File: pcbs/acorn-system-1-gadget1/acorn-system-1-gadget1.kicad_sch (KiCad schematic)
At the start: 13 parts, among them J2 DIN41612_02x32_AB_acorn-syste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

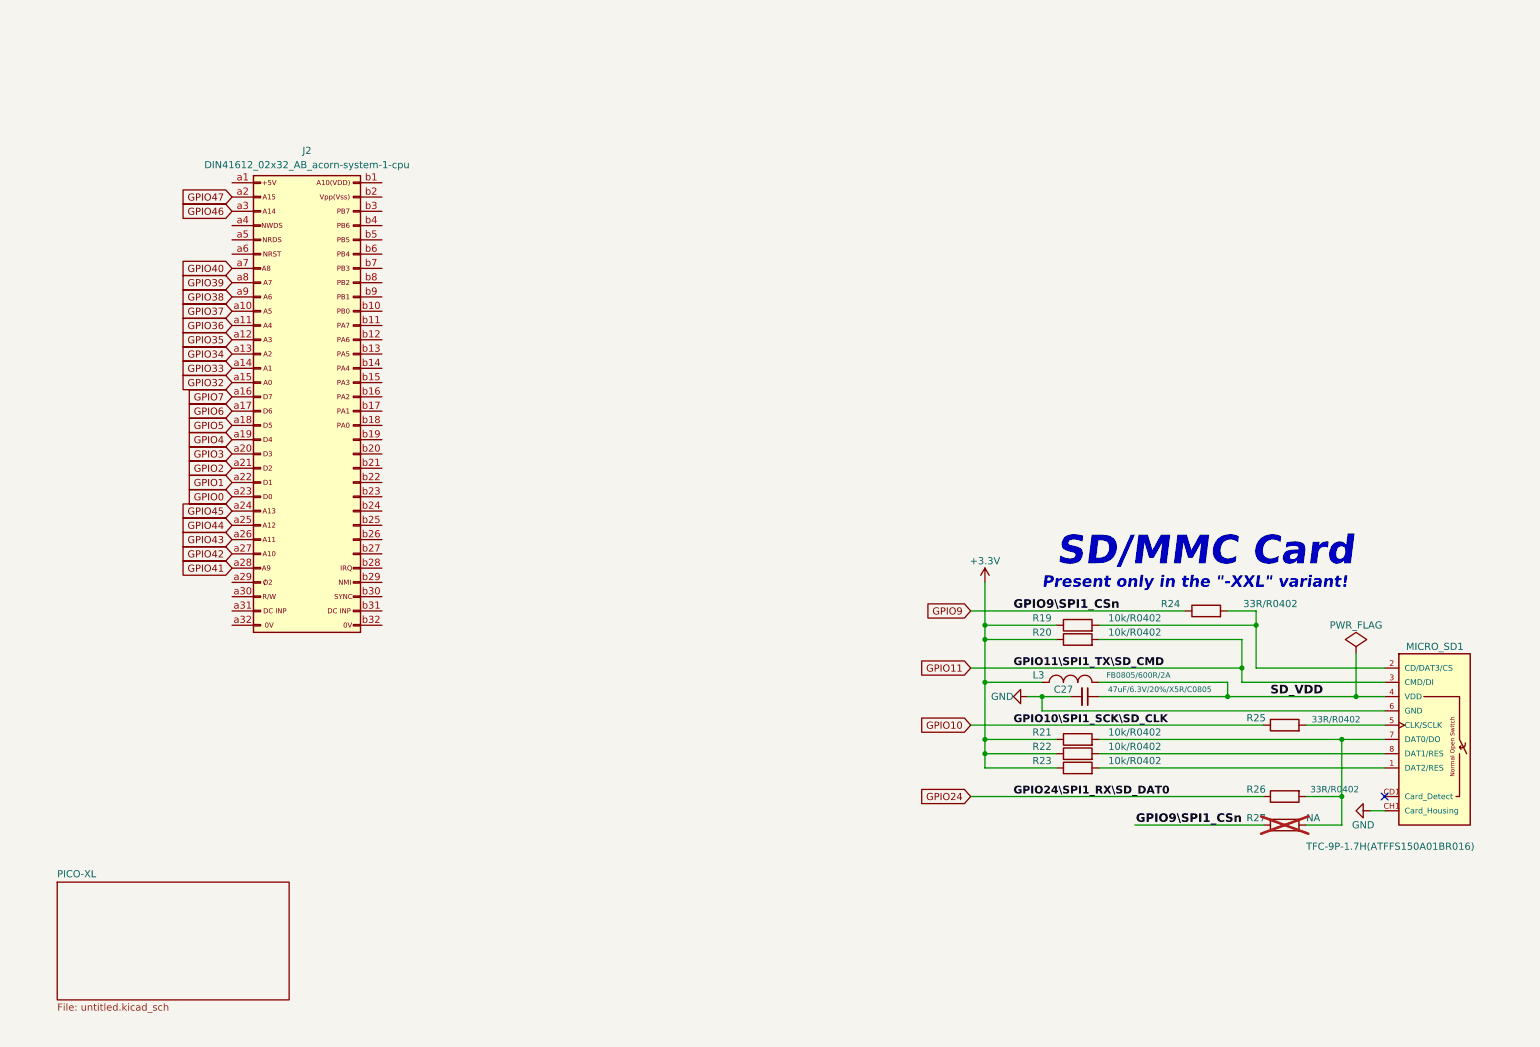
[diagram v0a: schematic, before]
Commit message: "Update"
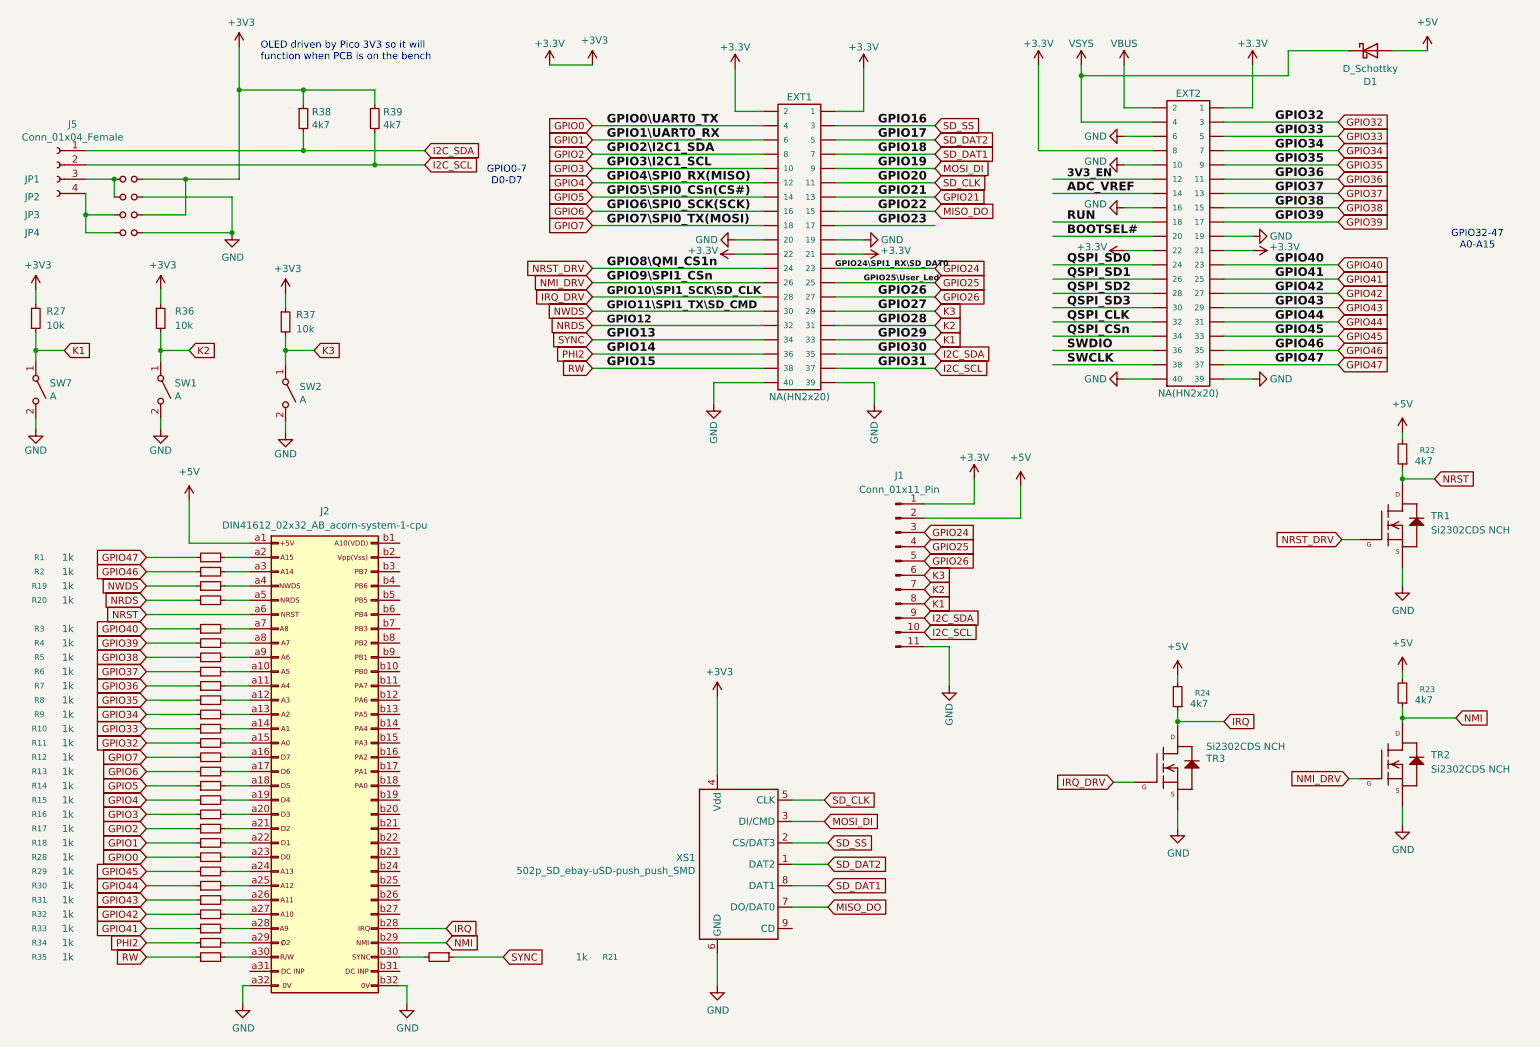
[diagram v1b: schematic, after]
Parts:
- removed C27: 47uF/6.3V/20%/X5R/C0805, OLIMEX_RLC-FP:C_0805_5MIL_DWS, symbol OLIMEX_RCL:C
- removed L3: FB0805/600R/2A, OLIMEX_RLC-FP:L_0805_5MIL_DWS, symbol OLIMEX_RCL:L
- removed MICRO_SD1: TFC-9P-1.7H(ATFFS150A01BR016), OLIMEX_Connectors-FP:uSD(TFC-9P-1.xH(ATFFS150A01BR016)), symbol OLIMEX_Connectors:MICRO_SD(TFC-9P-1.xH(ATFFS150A01BR016))
- removed R19, R20, R21, R22, R23: 10k/R0402, OLIMEX_RLC-FP:R_0402_5MIL_DWS, symbol OLIMEX_RCL:R
- removed R24, R25, R26: 33R/R0402, OLIMEX_RLC-FP:R_0402_5MIL_DWS, symbol OLIMEX_RCL:R
- removed R27: NA, OLIMEX_RLC-FP:R_0402_5MIL_DWS, symbol OLIMEX_RCL:R
- added D1: D_Schottky, Diode_SMD:D_SOD-123, symbol Device:D_Schottky
- added EXT1, EXT2: NA(HN2x20), Connector_PinSocket_2.54mm:PinSocket_2x20_P2.54mm_Vertical, symbol OLIMEX_Connectors:BH40S
- added J1: Conn_01x11_Pin, Connector_PinSocket_2.54mm:PinSocket_1x11_P2.54mm_Vertical, symbol Connector:Conn_01x11_Pin
- added J5: Conn_01x04_Female, Connector_PinHeader_2.54mm:PinHeader_1x04_P2.54mm_Vertical, symbol Connector:Conn_01x04_Female
- added JP1, JP2, JP3, JP4: Jumper_NO_Small, Jumper:SolderJumper-2_P1.3mm_Open_TrianglePad1.0x1.5mm, symbol Device:Jumper_NO_Small
- added R1, R10, R11, R12, R13, R14, R15, R16, R17, R18, R19, R2, R20, R21, R28, R29, R3, R30, R31, R32, R33, R34, R35, R4, R5, R6, R7, R8, R9: 1k, Resistor_SMD:R_0805_2012Metric_Pad1.20x1.40mm_HandSolder, symbol Device:R_Small
- added R22, R23, R24, R38, R39: 4k7, Resistor_SMD:R_0805_2012Metric_Pad1.20x1.40mm_HandSolder, symbol Device:R_Small
- added R27, R36, R37: 10k, Resistor_SMD:R_0805_2012Metric, symbol Device:R_Small
- added SW1, SW2, SW7: A, Button_Switch_THT:SW_PUSH_6mm, symbol mirotan-due-cassette-shield-cache:Switch_SW_SPST
- added TR1, TR2, TR3: Si2302CDS NCH, Package_TO_SOT_SMD:SOT-23, symbol ajm:Si2302CDS-n-channel
- added XS1: 502p_SD_ebay-uSD-push_push_SMD, ajm-acorn:Conn_uSDcard, symbol pico-9000-pack-rescue:502p_SD_ebay-uSD-push_push_SMD-pak_breakout
- J2: footprint Connector_DIN:DIN41612_R_2x32_Female_Horizontal_THT -> ajm-acorn:DIN41612_Q_2x32_Female_Horizontal_THT
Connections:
- net +3.3V: now also EXT1.1, EXT1.2, EXT1.21, EXT1.22, EXT2.1, EXT2.21, EXT2.22, EXT2.8, J1.1 (Pin_1), JP1.2, JP3.2, R27.1, R36.1, R37.1, R38.1, R39.1, XS1.4 (Vdd)
- net GND: now also J2.a32 (Pin_a32), J2.b32 (Pin_b32), EXT1.19, EXT1.20, EXT1.39, EXT1.40, EXT2.10, EXT2.16, EXT2.19, EXT2.39, EXT2.40, EXT2.6, J1.11 (Pin_11), JP2.2, JP4.2, SW1.2 (B), SW2.2 (B), SW7.2 (B), TR1.2 (S), TR2.2 (S), TR3.2 (S), XS1.6 (GND)
- net GPIO0: now also EXT1.4, R28.1; no longer J2.a23 (Pin_a23)
- net GPIO1: now also EXT1.6, R18.1; no longer J2.a22 (Pin_a22)
- net GPIO2: now also EXT1.8, R17.1; no longer J2.a21 (Pin_a21)
- net GPIO24: now also EXT1.23, J1.3 (Pin_3)
- net GPIO3: now also EXT1.10, R16.1; no longer J2.a20 (Pin_a20)
- net GPIO32: now also EXT2.3, R11.1; no longer J2.a15 (Pin_a15)
- net GPIO33: now also EXT2.5, R10.1; no longer J2.a14 (Pin_a14)
- net GPIO34: now also EXT2.7, R9.1; no longer J2.a13 (Pin_a13)
- net GPIO35: now also EXT2.9, R8.1; no longer J2.a12 (Pin_a12)
- net GPIO36: now also EXT2.11, R7.1; no longer J2.a11 (Pin_a11)
- net GPIO37: now also EXT2.13, R6.1; no longer J2.a10 (Pin_a10)
- net GPIO38: now also EXT2.15, R5.1; no longer J2.a9 (Pin_a9)
- net GPIO39: now also EXT2.17, R4.1; no longer J2.a8 (Pin_a8)
- net GPIO4: now also EXT1.12, R15.1; no longer J2.a19 (Pin_a19)
- net GPIO40: now also EXT2.23, R3.1; no longer J2.a7 (Pin_a7)
- net GPIO41: now also EXT2.25, R33.1; no longer J2.a28 (Pin_a28)
- net GPIO42: now also EXT2.27, R32.1; no longer J2.a27 (Pin_a27)
- net GPIO43: now also EXT2.29, R31.1; no longer J2.a26 (Pin_a26)
- net GPIO44: now also EXT2.31, R30.1; no longer J2.a25 (Pin_a25)
- net GPIO45: now also EXT2.33, R29.1; no longer J2.a24 (Pin_a24)
- net GPIO46: now also EXT2.35, R2.1; no longer J2.a3 (Pin_a3)
- net GPIO47: now also EXT2.37, R1.1; no longer J2.a2 (Pin_a2)
- net GPIO5: now also EXT1.14, R14.1; no longer J2.a18 (Pin_a18)
- net GPIO6: now also EXT1.16, R13.1; no longer J2.a17 (Pin_a17)
- net GPIO7: now also EXT1.18, R12.1; no longer J2.a16 (Pin_a16)
- net +5V: now reaches J2.a1 (Pin_a1)
- net +5V: now also D1.2 (A), J1.2 (Pin_2), R22.2, R23.2, R24.2
- net at J2.a29 (Pin_a29): now also R34.2
- net at J2.a30 (Pin_a30): now also R35.2
- net at J2.a4 (Pin_a4): now also R19.2
- net at J2.a5 (Pin_a5): now also R20.2
- net NRST: now reaches J2.a6 (Pin_a6)
- net NRST: now also R22.1, TR1.3 (D)
- net IRQ: now reaches J2.b28 (Pin_b28)
- net IRQ: now also R24.1, TR3.3 (D)
- net NMI: now reaches J2.b29 (Pin_b29)
- net NMI: now also R23.1, TR2.3 (D)
- net at J2.b30 (Pin_b30): now also R21.2
- new net: J5.3 (Pin_3), JP1.1, JP2.1
- new net: J5.4 (Pin_4), JP3.1, JP4.1
- new net: J2.a11 (Pin_a11), R7.2
- new net: J2.a12 (Pin_a12), R8.2
- new net: J2.a23 (Pin_a23), R28.2
- new net: J2.a16 (Pin_a16), R12.2
- new net: J2.a10 (Pin_a10), R6.2
- new net: J2.a19 (Pin_a19), R15.2
- new net: J2.a3 (Pin_a3), R2.2
- new net: J2.a13 (Pin_a13), R9.2
- new net: J2.a14 (Pin_a14), R10.2
- new net: J2.a15 (Pin_a15), R11.2
- new net: J2.a17 (Pin_a17), R13.2
- new net: J2.a18 (Pin_a18), R14.2
- new net: J2.a2 (Pin_a2), R1.2
- new net: J2.a20 (Pin_a20), R16.2
- new net: J2.a21 (Pin_a21), R17.2
- new net: J2.a22 (Pin_a22), R18.2
- new net: J2.a24 (Pin_a24), R29.2
- new net: J2.a25 (Pin_a25), R30.2
- new net: J2.a26 (Pin_a26), R31.2
- new net: J2.a27 (Pin_a27), R32.2
- new net: J2.a28 (Pin_a28), R33.2
- new net: J2.a7 (Pin_a7), R3.2
- new net: J2.a8 (Pin_a8), R4.2
- new net: J2.a9 (Pin_a9), R5.2
- new net 3V3_EN: EXT2.12
- new net ADC_VREF: EXT2.14
- new net BOOTSEL#: EXT2.20
- new net GPIO21: EXT1.13
- new net GPIO23: EXT1.17
- new net GPIO25: EXT1.25, J1.4 (Pin_4)
- new net GPIO26: EXT1.27, J1.5 (Pin_5)
- new net I2C_SCL: EXT1.37, J1.10 (Pin_10), J5.2 (Pin_2), R39.2
- new net I2C_SDA: EXT1.35, J1.9 (Pin_9), J5.1 (Pin_1), R38.2
- new net IRQ_DRV: EXT1.28, TR3.1 (G)
- new net K1: EXT1.33, J1.8 (Pin_8), R27.2, SW7.1 (A)
- new net K2: EXT1.31, J1.7 (Pin_7), R36.2, SW1.1 (A)
- new net K3: EXT1.29, J1.6 (Pin_6), R37.2, SW2.1 (A)
- new net MISO_DO: EXT1.15, XS1.7 (DO/DAT0)
- new net MOSI_DI: EXT1.9, XS1.3 (DI/CMD)
- new net NMI_DRV: EXT1.26, TR2.1 (G)
- new net NRDS: EXT1.32, R20.1
- new net NRST_DRV: EXT1.24, TR1.1 (G)
- new net NWDS: EXT1.30, R19.1
- new net PHI2: EXT1.36, R34.1
- new net QSPI_CLK: EXT2.32
- new net QSPI_CSn: EXT2.34
- new net QSPI_SD0: EXT2.24
- new net QSPI_SD1: EXT2.26
- new net QSPI_SD2: EXT2.28
- new net QSPI_SD3: EXT2.30
- new net RUN: EXT2.18
- new net RW: EXT1.38, R35.1
- new net SD_CLK: EXT1.11, XS1.5 (CLK)
- new net SD_DAT1: EXT1.7, XS1.8 (DAT1)
- new net SD_DAT2: EXT1.5, XS1.1 (DAT2)
- new net SD_SS: EXT1.3, XS1.2 (CS/DAT3)
- new net SWCLK: EXT2.38
- new net SWDIO: EXT2.36
- new net SYNC: EXT1.34, R21.1
- new net VBUS: EXT2.2
- new net VSYS: D1.1 (K), EXT2.4
- no-connect marks 1 -> 0
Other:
- removed sheet PICO-XL
- note added: "GPIO0-7 D0-D7"
- note added: "GPIO32-47 A0-A15"
- note added: "OLED driven by Pico 3V3 so it will function when PCB is on the bench"
- note removed: "Present only in the "-XXL" variant!"
- note removed: "SD/MMC Card"
- moved on the sheet: J2

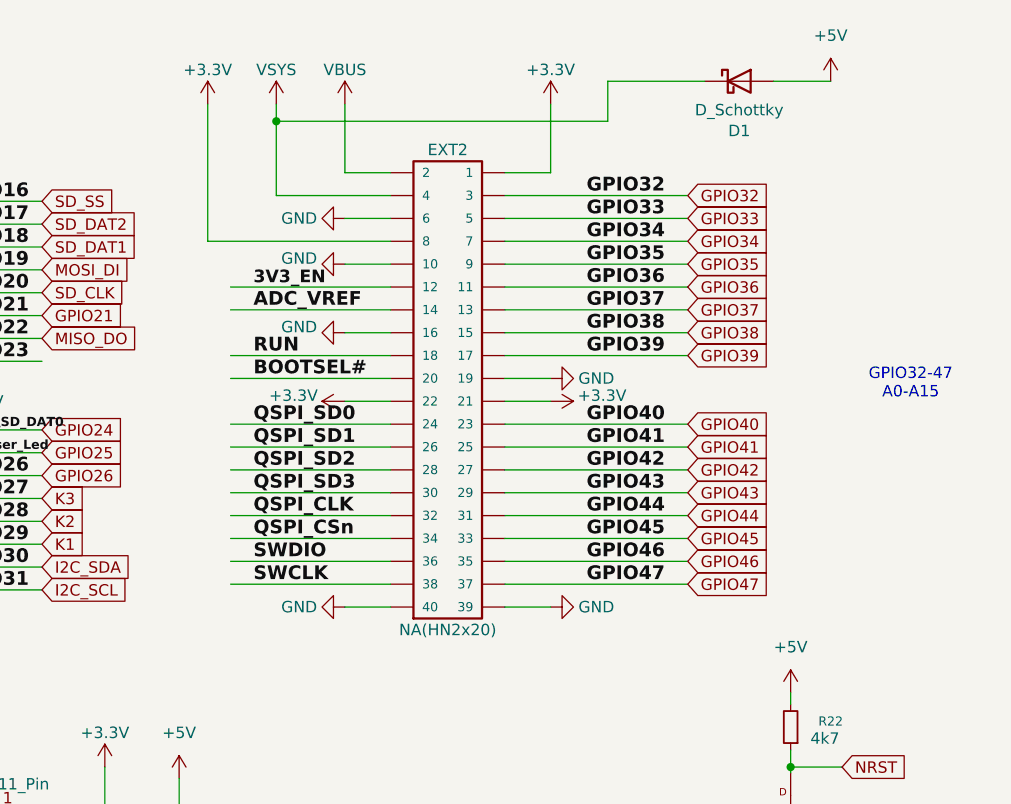
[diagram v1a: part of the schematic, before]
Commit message: "Update"
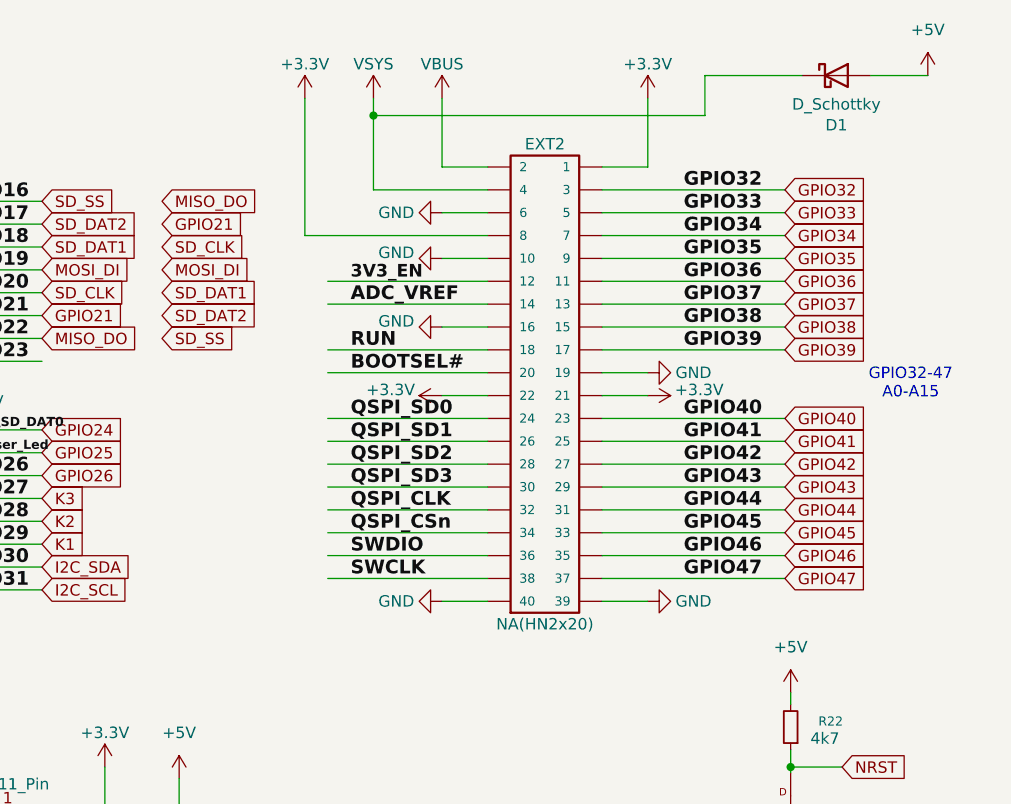
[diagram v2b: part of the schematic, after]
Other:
- moved on the sheet: D1, EXT2
